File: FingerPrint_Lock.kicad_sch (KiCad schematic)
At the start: 13 parts, among them J1 Fingerprint Sensor, J2 12V Solenoid Lock, J3 12V Relay, SW1 Button1, SW2 Button2, SW3 Button3, SW4 Button4, U2 I2C 2X16 LCD

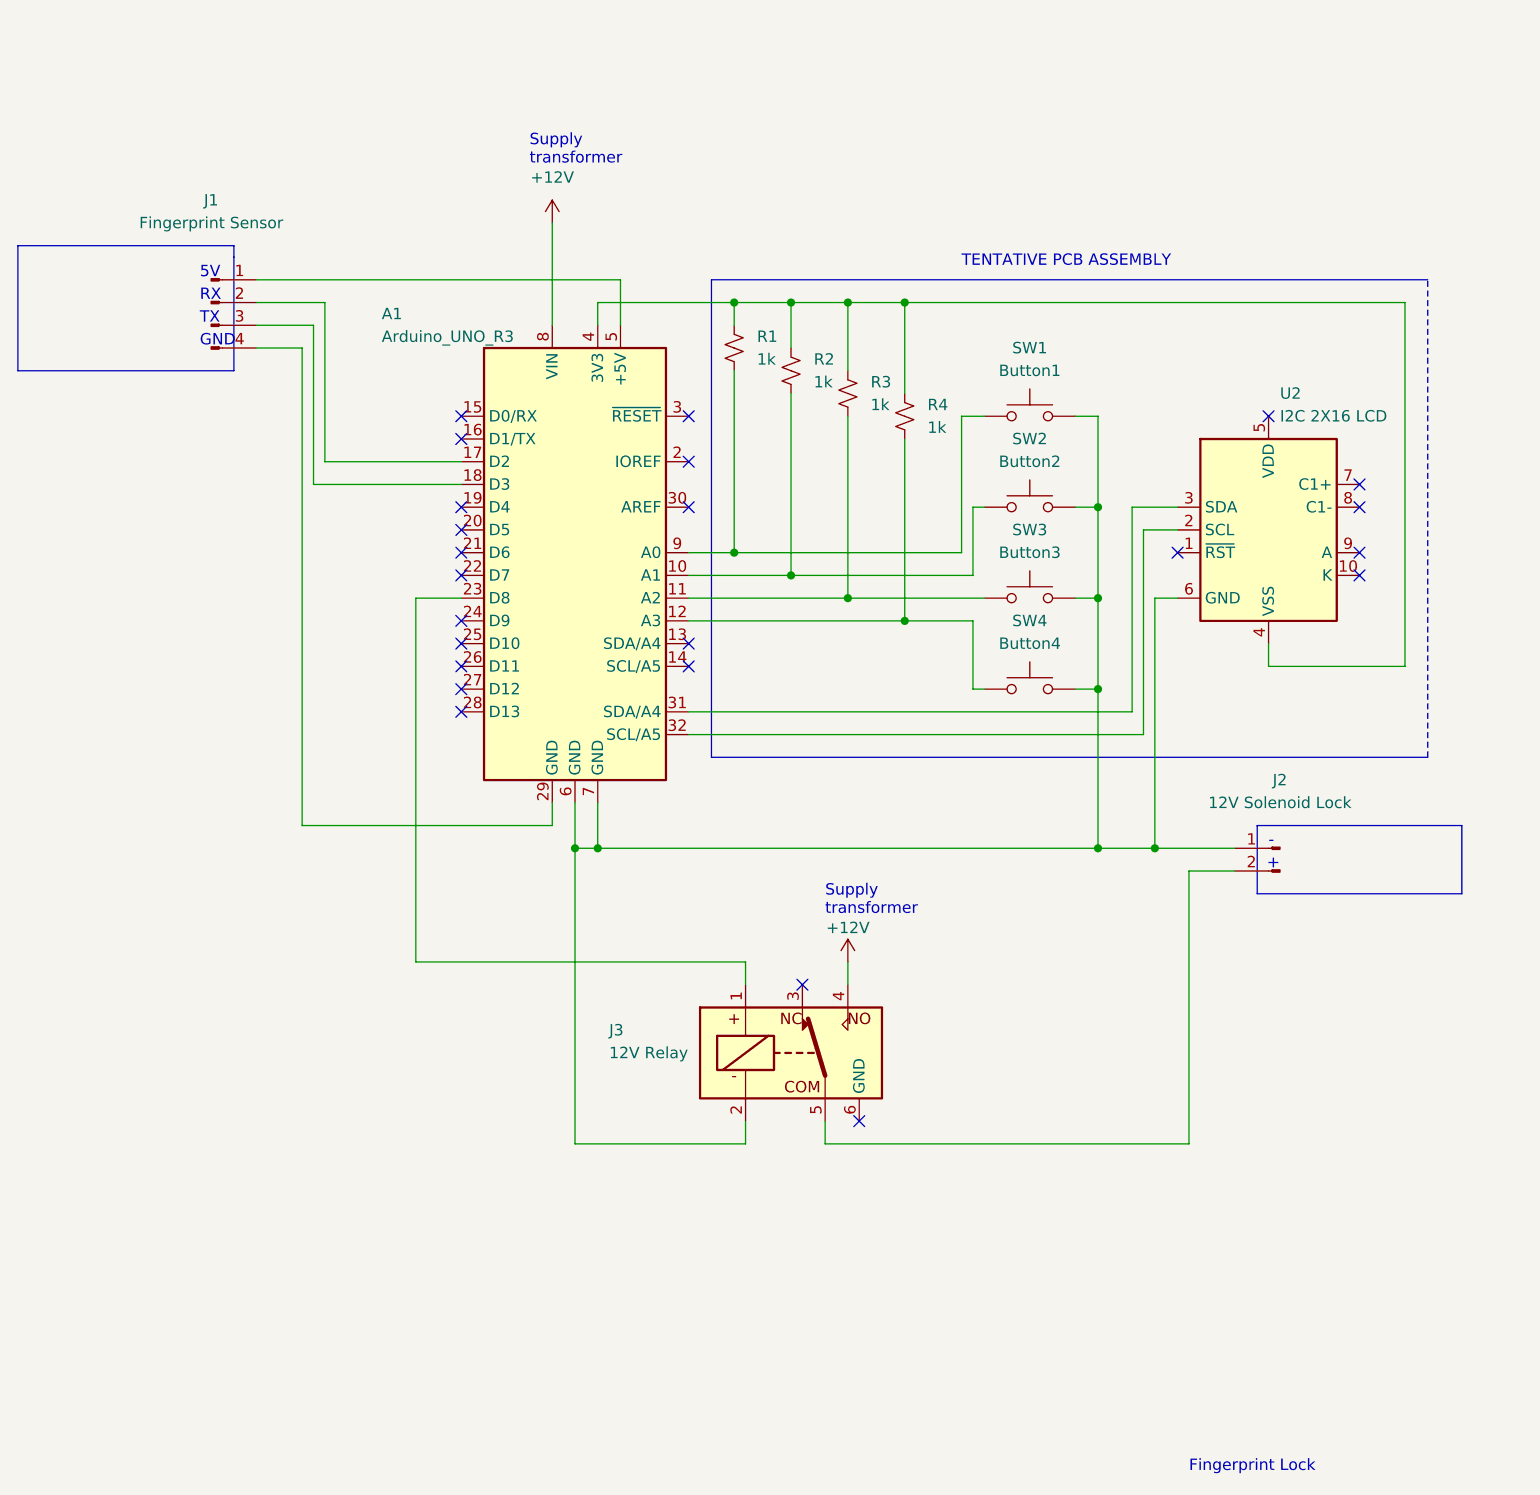
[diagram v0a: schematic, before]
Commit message: Final(?) schematics/PCB upload
Final(?) version of overview schematic, PCB file, and PCB Schematic.
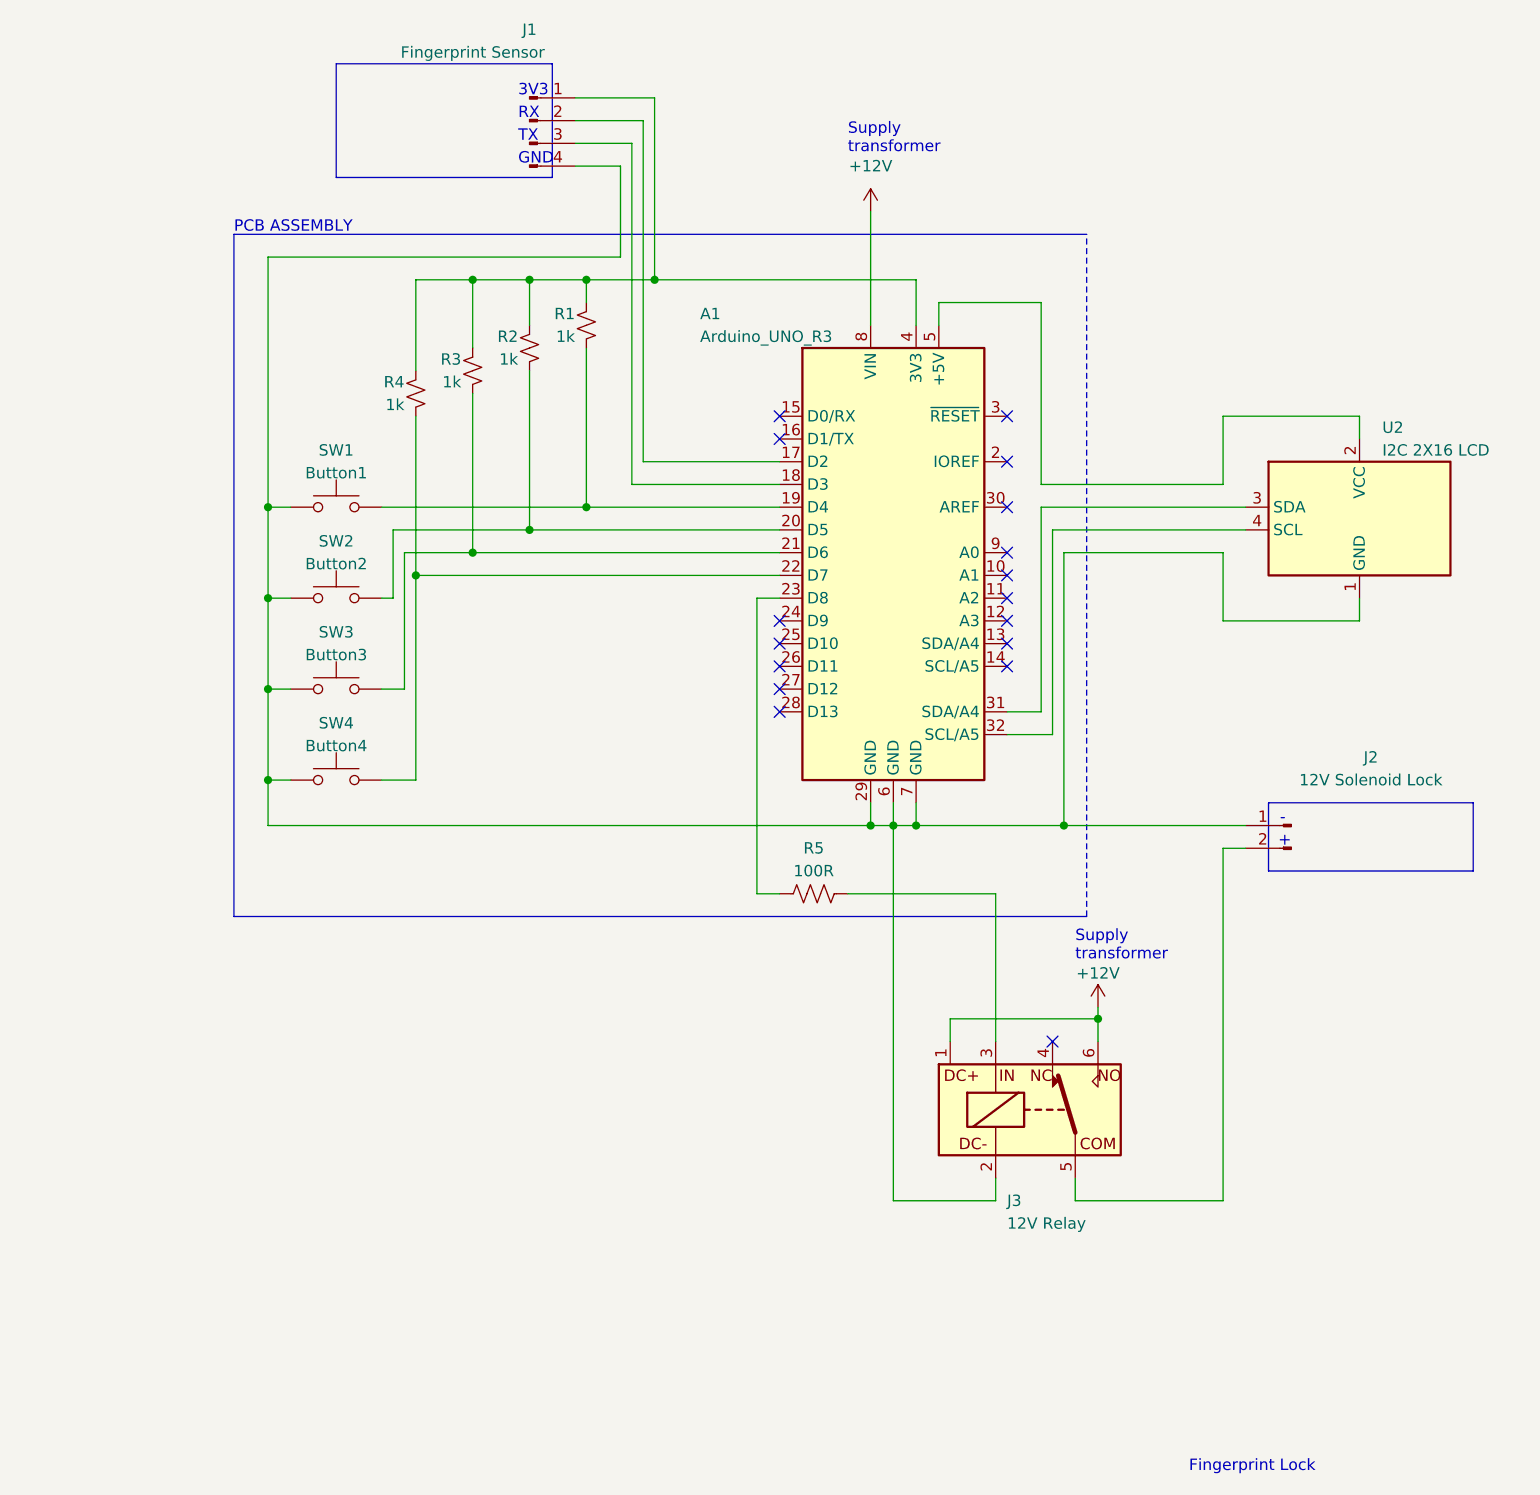
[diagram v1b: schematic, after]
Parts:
- added R5: 100R, symbol Device:R_US
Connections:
- net +12V: now also J3.1, J3.6; no longer J3.4
- net at A1.4 (3V3), R1.1, R2.1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: now also J1.1 (Pin_1); no longer U2.4 (VSS)
- net at R2.2, SW2.1: now also A1.20 (D5); no longer A1.10 (A1)
- net at A1.5 (+5V): now also U2.2 (VCC); no longer J1.1 (Pin_1)
- net at A1.29 (GND), J1.4 (Pin_4): now also A1.6 (GND), A1.7 (GND), J2.1 (Pin_1), J3.2, SW1.2, SW2.2, SW3.2, SW4.2, U2.1 (GND)
- net at A1.23 (D8): now also R5.1; no longer J3.1
- net at J3.3: now also R5.2
- net at R1.2, SW1.1: now also A1.19 (D4); no longer A1.9 (A0)
- net at R4.2, SW4.1: now also A1.22 (D7); no longer A1.12 (A3)
- net at R3.2, SW3.1: now also A1.21 (D6); no longer A1.11 (A2)
- net at A1.32 (SCL/A5): now also U2.4 (SCL); no longer U2.2 (SCL)
- no-connect marks 24 -> 17
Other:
- note added: "3V3"
- note added: "PCB ASSEMBLY"
- note removed: "5V"
- note removed: "TENTATIVE PCB ASSEMBLY"
- moved on the sheet: A1, J1, J2, J3, R1, R2, R3, R4, SW1, SW2, SW3, SW4
